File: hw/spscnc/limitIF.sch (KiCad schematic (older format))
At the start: 20 parts, among them J20 8P8C_4xShielded, J5 Limit_IF

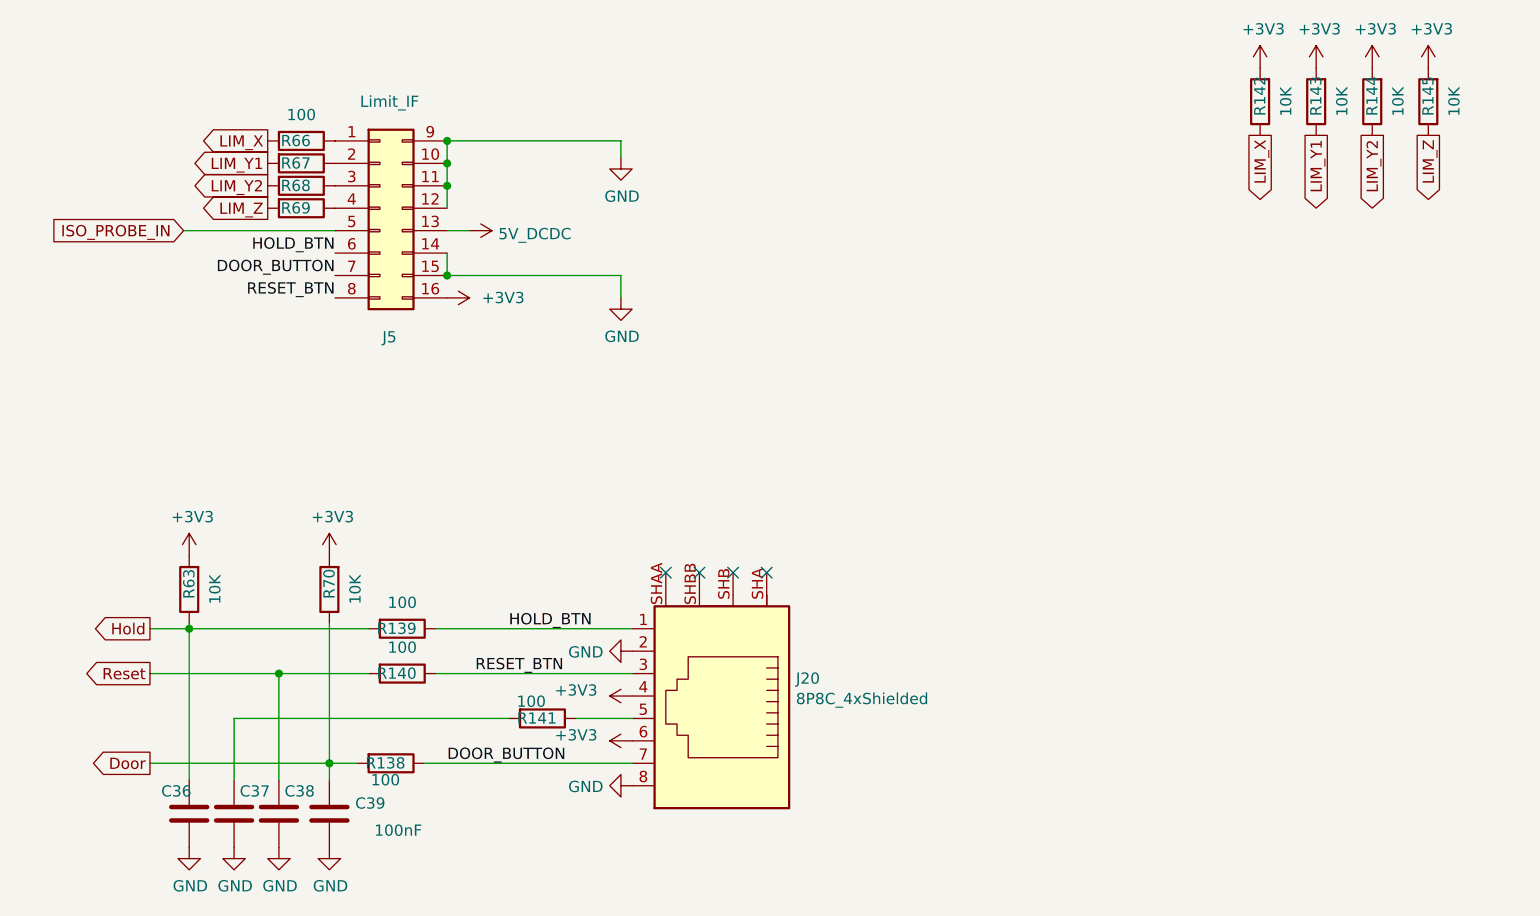
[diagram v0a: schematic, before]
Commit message: Finished preliminary routing, pending checklist and review
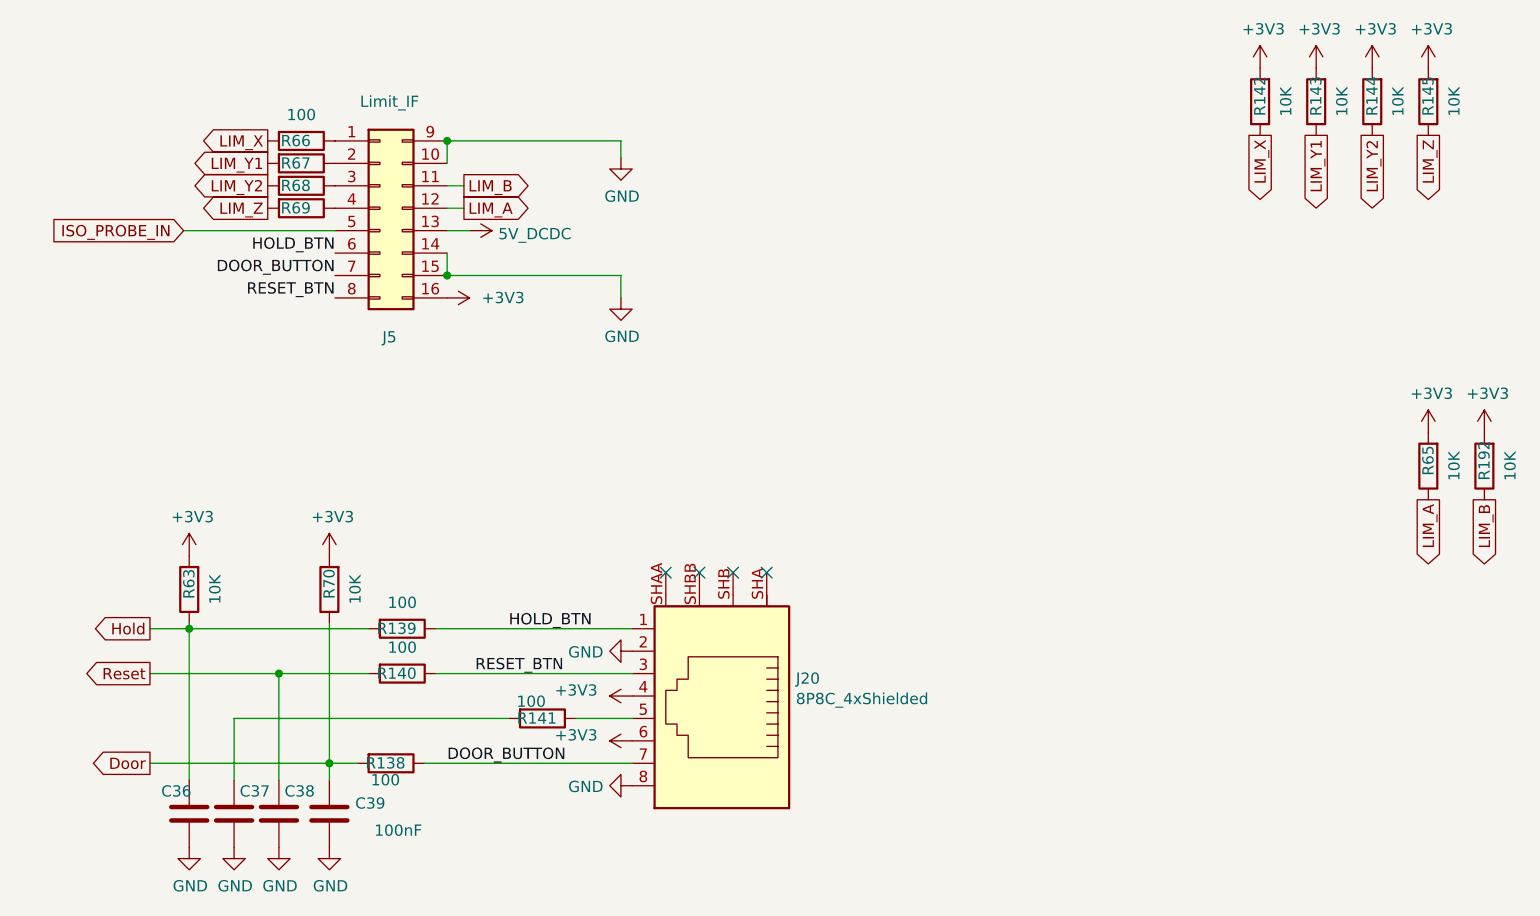
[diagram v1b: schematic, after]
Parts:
- added R192, R65: 10K, Resistor_SMD:R_0805_2012Metric, symbol Device:R
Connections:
- net +3V3: now also R192.2, R65.2
- net GND: no longer J5.11 (Pin_11), J5.12 (Pin_12)
- new net LIM_A: J5.12 (Pin_12), R65.1
- new net LIM_B: J5.11 (Pin_11), R192.1
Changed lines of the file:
@@
 $EndComp
-Wire Wire Line
-	3825 3775 3825 3675
 Wire Wire Line
 	3825 3675 3825 3575
-Connection ~ 3825 3675
 Wire Wire Line
 	3825 3575 4600 3575
@@
 Wire Wire Line
 	3925 3975 3825 3975
-Wire Wire Line
-	3825 3875 3825 3775
-Connection ~ 3825 3775
 $Comp
 L industrial:8P8C_4xShielded J?
@@
 Text Label 3325 4275 2    50   ~ 0
 RESET_BTN
+Text GLabel 8450 5175 3    50   Output ~ 0
+LIM_B
+Text GLabel 8200 5175 3    50   Output ~ 0
+LIM_A
+$Comp
+L Device:R R?
+U 1 1 62172151
+P 8200 5025
+AR Path="/61C80DFB/62172151" Ref="R?"  Part="1"
+AR Path="/61C80E48/62172151" Ref="R?"  Part="1"
+AR Path="/61C80E8F/62172151" Ref="R?"  Part="1"
+AR Path="/61CEF4C9/62172151" Ref="R?"  Part="1"
+AR Path="/61E6D951/62172151" Ref="R65"  Part="1"
+F 0 "R65" V 8200 5000 50  0000 C CNN
+F 1 "10K" V 8084 5025 50  0000 C CNN
+F 2 "Resistor_SMD:R_0805_2012Metric" V 8130 5025 50  0001 C CNN
+F 3 "~" H 8200 5025 50  0001 C CNN
+F 4 "C17414" H 8200 5025 50  0001 C CNN "jlcpcb"
+	1    8200 5025
+	-1   0    0    1
+$EndComp
+$Comp
+L industrial:+3V3 #PWR?
+U 1 1 6217215B
+P 8200 4875
+AR Path="/61C80DFB/6217215B" Ref="#PWR?"  Part="1"
+AR Path="/61C80E48/6217215B" Ref="#PWR?"  Part="1"
+AR Path="/61C80E8F/6217215B" Ref="#PWR?"  Part="1"
+AR Path="/61CEF4C9/6217215B" Ref="#PWR?"  Part="1"
+AR Path="/61E6D951/6217215B" Ref="#PWR0169"  Part="1"
+F 0 "#PWR0169" H 8200 4725 50  0001 C CNN
+F 1 "+3V3" H 8215 5048 50  0000 C CNN
+F 2 "" H 8200 4875 50  0001 C CNN
+F 3 "" H 8200 4875 50  0001 C CNN
+	1    8200 4875
+	1    0    0    -1
+$EndComp
+$Comp
+L Device:R R?
+U 1 1 62172166
+P 8450 5025
+AR Path="/61C80DFB/62172166" Ref="R?"  Part="1"
+AR Path="/61C80E48/62172166" Ref="R?"  Part="1"
+AR Path="/61C80E8F/62172166" Ref="R?"  Part="1"
+AR Path="/61CEF4C9/62172166" Ref="R?"  Part="1"
+AR Path="/61E6D951/62172166" Ref="R192"  Part="1"
+F 0 "R192" V 8450 5000 50  0000 C CNN
+F 1 "10K" V 8334 5025 50  0000 C CNN
+F 2 "Resistor_SMD:R_0805_2012Metric" V 8380 5025 50  0001 C CNN
+F 3 "~" H 8450 5025 50  0001 C CNN
+F 4 "C17414" H 8450 5025 50  0001 C CNN "jlcpcb"
+	1    8450 5025
+	-1   0    0    1
+$EndComp
+$Comp
+L industrial:+3V3 #PWR?
+U 1 1 62172170
+P 8450 4875
+AR Path="/61C80DFB/62172170" Ref="#PWR?"  Part="1"
+AR Path="/61C80E48/62172170" Ref="#PWR?"  Part="1"
+AR Path="/61C80E8F/62172170" Ref="#PWR?"  Part="1"
+AR Path="/61CEF4C9/62172170" Ref="#PWR?"  Part="1"
+AR Path="/61E6D951/62172170" Ref="#PWR0170"  Part="1"
+F 0 "#PWR0170" H 8450 4725 50  0001 C CNN
+F 1 "+3V3" H 8465 5048 50  0000 C CNN
+F 2 "" H 8450 4875 50  0001 C CNN
+F 3 "" H 8450 4875 50  0001 C CNN
+	1    8450 4875
+	1    0    0    -1
+$EndComp
+Text GLabel 3900 3775 2    50   Output ~ 0
+LIM_B
+Text GLabel 3900 3875 2    50   Output ~ 0
+LIM_A
+Wire Wire Line
+	3900 3775 3825 3775
+Wire Wire Line
+	3825 3875 3900 3875
 $EndSCHEMATC
